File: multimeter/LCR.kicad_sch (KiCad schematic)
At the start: 16 parts, among them J301 Conn_01x01_Socket, J302 Conn_01x01_Socket, J303 Conn_01x01_Socket, U301 TMUX1108PW, U302 OPA4322AIPWR

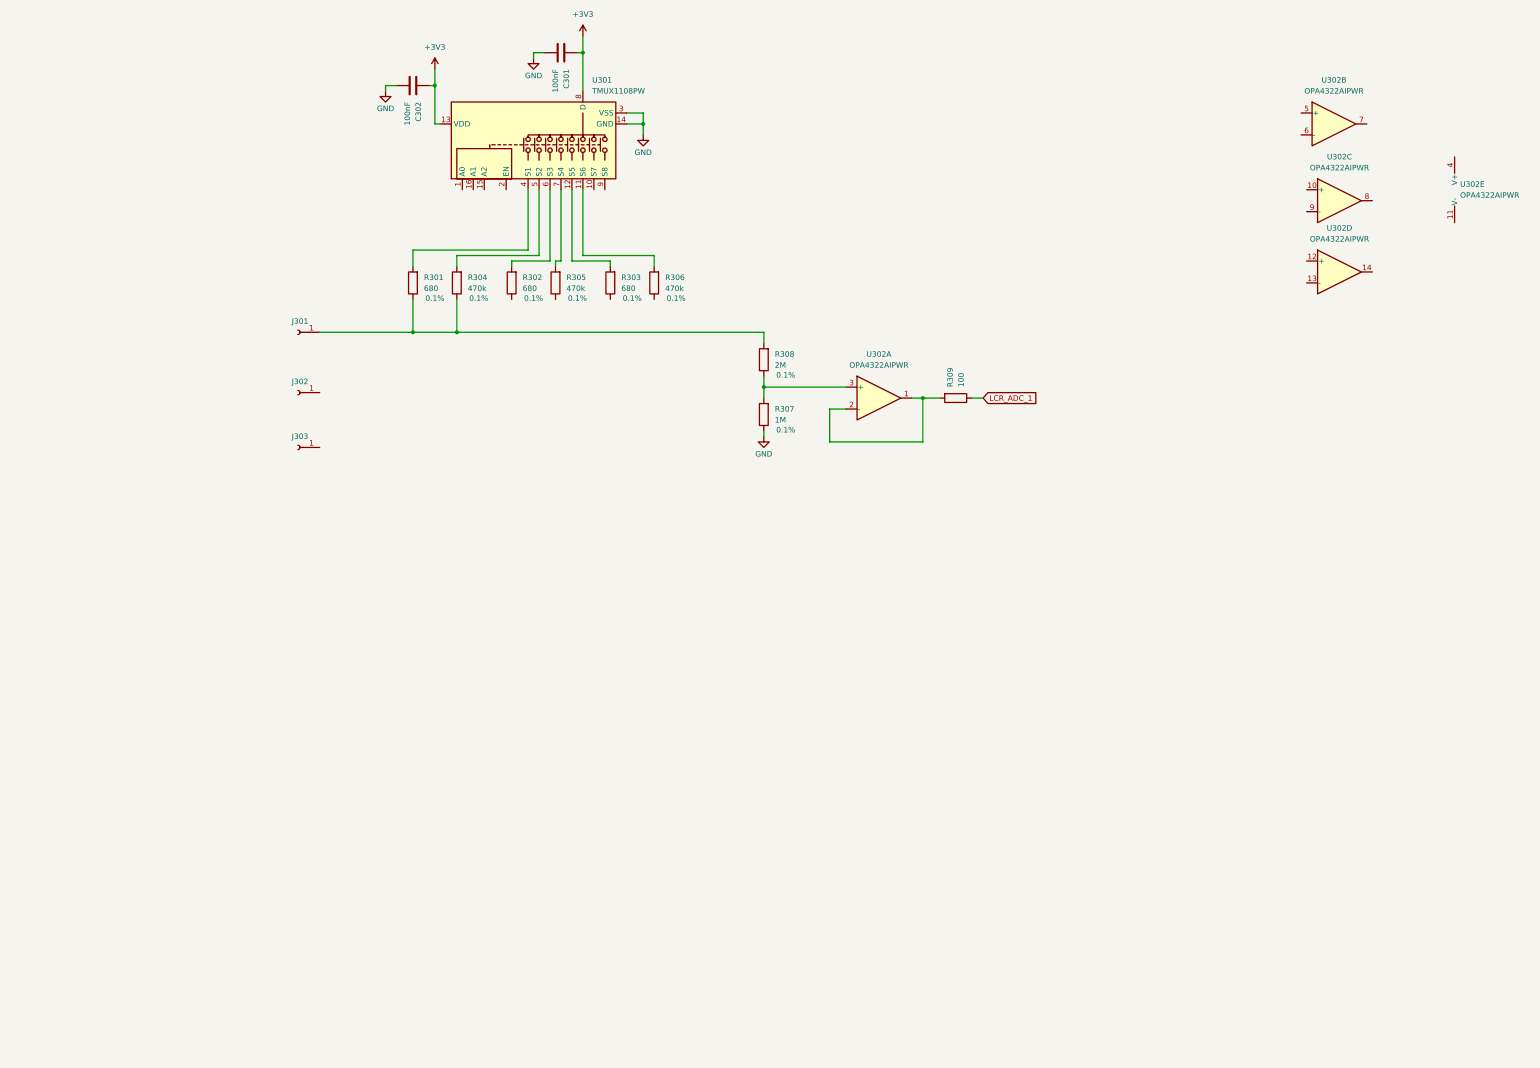
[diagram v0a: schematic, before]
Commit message: UPDATE
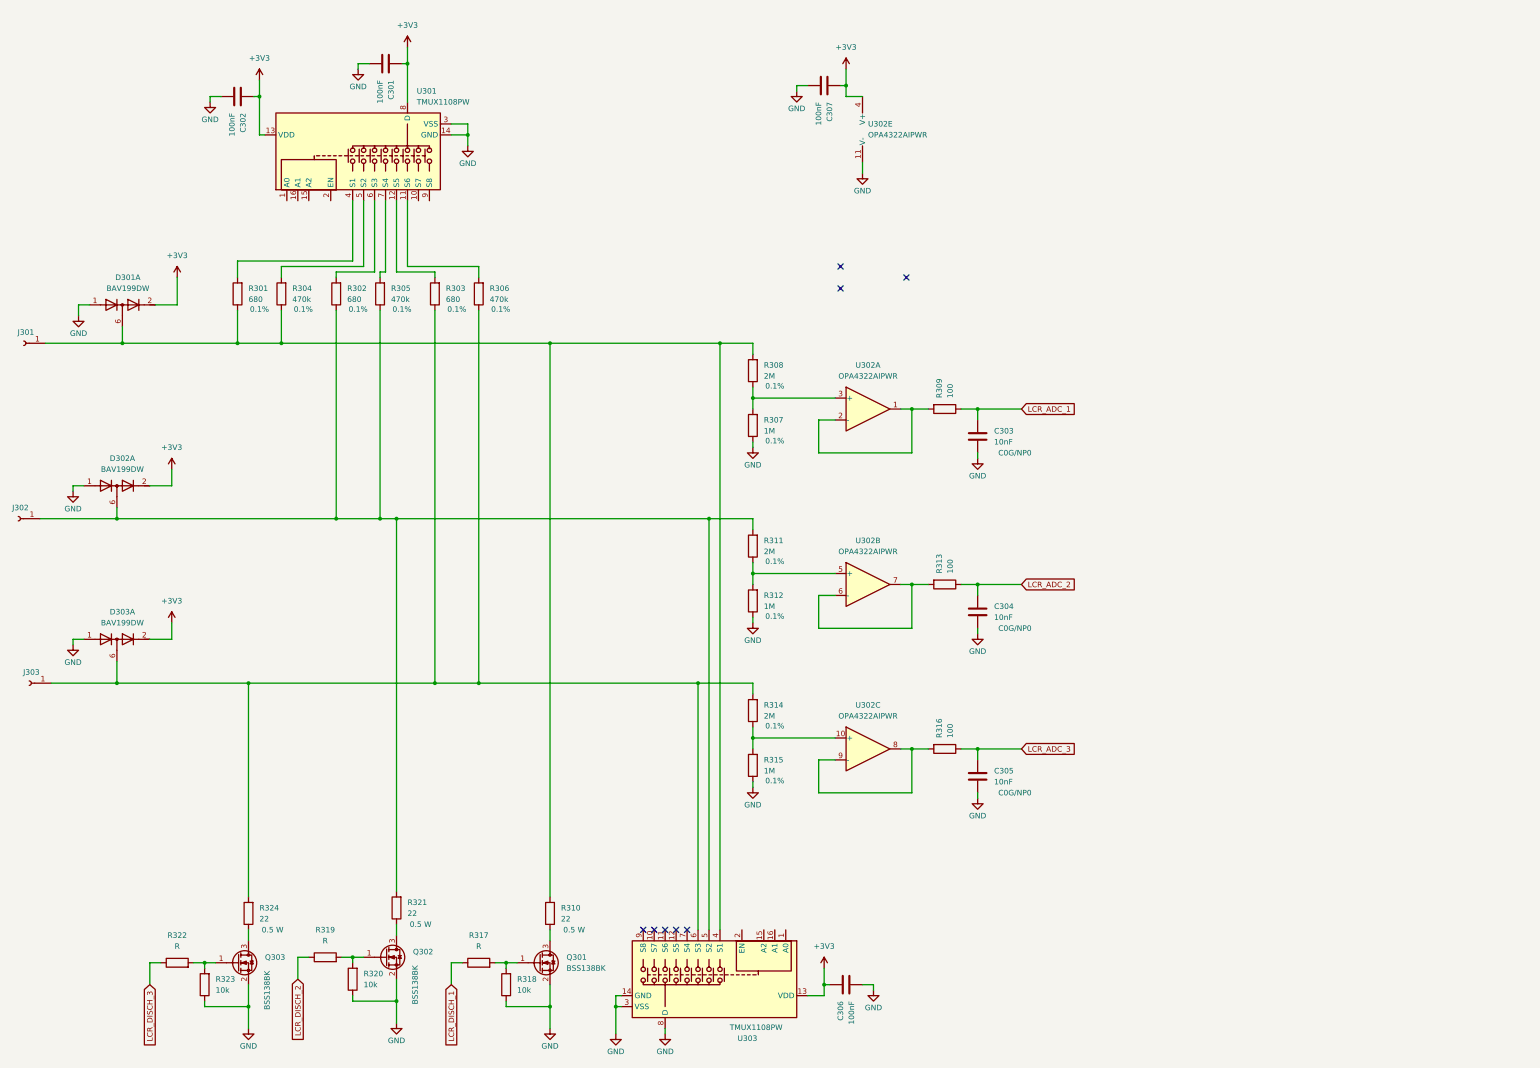
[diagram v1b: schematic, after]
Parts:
- removed unit 4 of U302
- added C303, C304, C305: 10nF, symbol Device:C
- added C306, C307: 100nF, symbol Device:C
- added D301, D302, D303: BAV199DW, Package_TO_SOT_SMD:SOT-363_SC-70-6, symbol Diode:BAV199DW
- added Q301, Q302, Q303: BSS138BK, Package_TO_SOT_SMD:SOT-23, symbol Transistor_FET:BSS138
- added R310, R321, R324: 22, symbol Device:R
- added R311, R314: 2M, symbol Device:R
- added R312, R315: 1M, symbol Device:R
- added R313, R316: 100, symbol Device:R
- added R317, R319, R322: R, symbol Device:R
- added R318, R320, R323: 10k, symbol Device:R
- added U303: TMUX1108PW, Package_SO:TSSOP-16_4.4x5mm_P0.65mm, symbol Analog_Switch:TMUX1108PW
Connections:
- net +3V3: now also U302.4 (V+), C306.1, C307.1, D301.2 (K2), D302.2 (K2), D303.2 (K2), U303.13 (VDD)
- net GND: now also U302.11 (V-), C303.2, C304.2, C305.2, C306.2, C307.2, D301.1 (A1), D302.1 (A1), D303.1 (A1), Q301.2 (S), Q302.2 (S), Q303.2 (S), R312.1, R315.1, R318.1, R320.1, R323.1, U303.14 (GND), U303.3 (VSS), U303.8 (D)
- net LCR_ADC_1: now also C303.1
- net at J301.1 (Pin_1), R301.1, R304.1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: now also D301.6 (K3A4), R310.2, U303.4 (S1)
- net at R302.1: now also J302.1 (Pin_1), R305.1, D302.6 (K3A4), R311.2, R321.2, U303.5 (S2)
- net at U302.10 (+): now also R314.1, R315.2
- net at U302.8: now also U302.9 (-), R316.2
- net at U302.5 (+): now also R311.1, R312.2
- net at U302.6 (-): now also U302.7, R313.2
- net at J303.1 (Pin_1): now also R303.1, R306.1, D303.6 (K3A4), R314.2, R324.2, U303.6 (S3)
- new net: Q302.3 (D), R321.1
- new net: Q302.1 (G), R319.2, R320.2
- new net: Q303.1 (G), R322.2, R323.2
- new net: Q301.1 (G), R317.2, R318.2
- new net: Q301.3 (D), R310.1
- new net: Q303.3 (D), R324.1
- new net LCR_ADC_2: C304.1, R313.1
- new net LCR_ADC_3: C305.1, R316.1
- new net LCR_DISCH_1: R317.1
- new net LCR_DISCH_2: R319.1
- new net LCR_DISCH_3: R322.1
- no-connect marks 0 -> 8
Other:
- moved on the sheet: C301, C302, J301, J302, J303, R301, R302, R303, R304, R305, R306, R307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
